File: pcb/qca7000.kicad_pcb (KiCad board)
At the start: 4 copper layers, 42.2 x 28.8 mm, 113 parts, among them J1 Conn_01x20, J2 JTAG, J3 FLASH, U1 AT25SF081-SSHD-X, Y1 25MHz

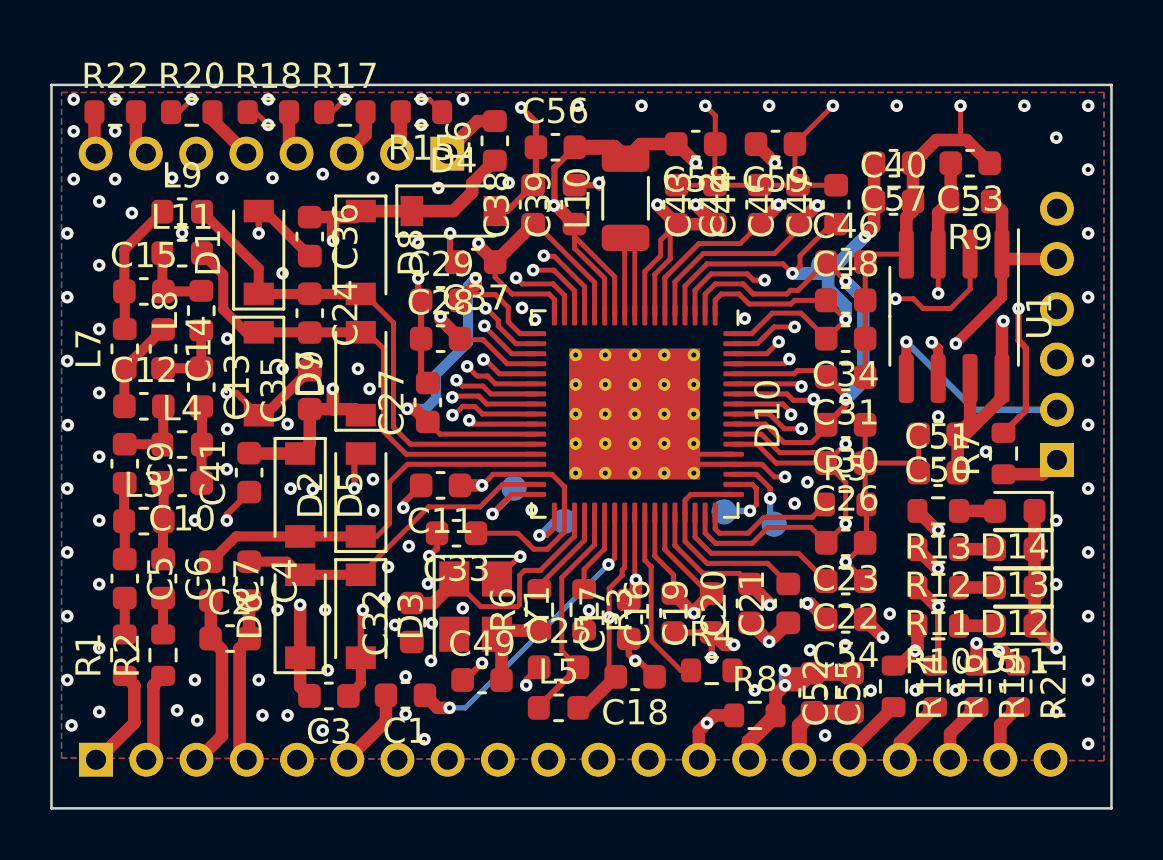
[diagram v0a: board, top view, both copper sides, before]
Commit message: v2, new filter, rbias
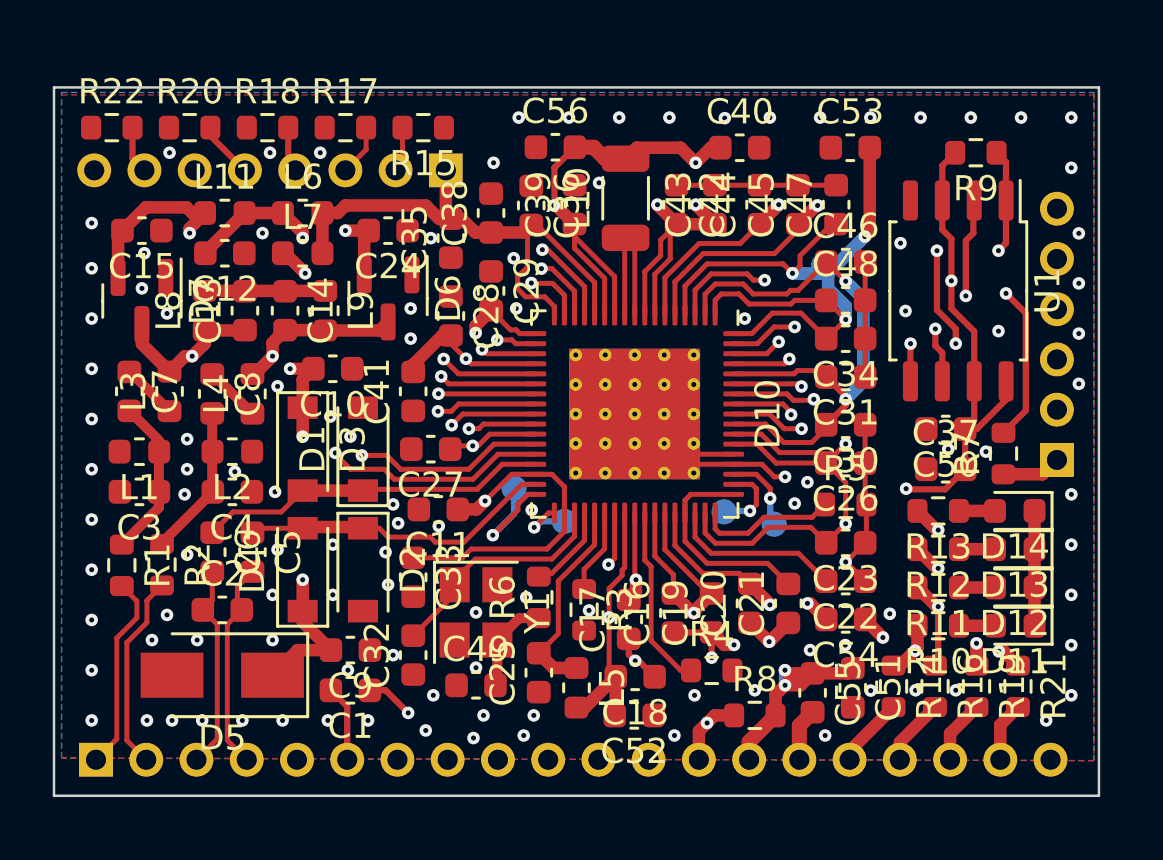
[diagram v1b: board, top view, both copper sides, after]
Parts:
- removed C57, C58, C59: 10uF 25V, Capacitor_SMD:C_0603_1608Metric
- removed D8, D9: 1N4148W, Diode_SMD:D_SOD-123
- added C8: 1.5nF, Capacitor_SMD:C_0603_1608Metric, F.Cu at (118.8, 61.0)
- added L1: 1.8uH, Inductor_SMD:L_0603_1608Metric, F.Cu at (115.9, 63.3)
- added L2: 1.8uH, Inductor_SMD:L_0603_1608Metric, F.Cu at (119.6, 63.3)
- C12, C35, C36, C37: value 100nF -> 10uF 25V
- C13, C14, C2, C3, C4: value 100nF -> 220pF
- C15, C24, C7: value 100nF -> 1.5nF
- C51: value 10uF 25V -> 100nF
- D1, D2, D3: value 1N4148W -> B5819W
- D4: value 4V7 -> B5819W
- D5: value 1N4148W -> 3V9; footprint Diode_SMD:D_SOD-123 -> Diode_SMD:D_SMA
- D6, D7: value 1N4148W -> BAV99; footprint Diode_SMD:D_SOD-123 -> Package_TO_SOT_SMD:SOT-23
- L11, L8, L9: value Bead 600 -> 1.8uH
- L3, L4: value Bead 600 -> 270nH
- R1, R2: value R_Small -> 22
- U1: value AT25SF081-SSHD-X -> 25Q16; footprint Package_SO:SOIC-8_3.9x4.9mm_P1.27mm -> Package_SO:SOP-8_5.28x5.23mm_P1.27mm
- moved C37 20.5 mm to (148.0, 64.0), turned to 0 degrees
- moved D4 15.5 mm to (122.4, 68.0), turned to 90 degrees
- moved D6 13.1 mm to (125.8, 57.2), turned to -90 degrees
- moved C9 11.7 mm to (124.3, 71.2), turned to 180 degrees
- moved C3 11.1 mm to (115.9, 64.9)
- moved C51 9.22 mm to (144.3, 72.7), turned to -90 degrees
- moved C36 8.90 mm to (131.5, 53.5)
- moved D1 8.86 mm to (124.8, 63.2)
- moved C52 8.72 mm to (135.6, 73.8), turned to 180 degrees
- moved C35 8.24 mm to (128.3, 54.8)
- moved C7 8.22 mm to (115.5, 60.9)
- moved L6 8.17 mm to (122.4, 53.8), turned to 0 degrees
- moved L7 8.04 mm to (122.4, 55.4), turned to 0 degrees
- moved D5 7.82 mm to (119.2, 72.2), turned to 180 degrees
- moved C10 7.52 mm to (123.6, 60.0)
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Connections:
- C10 pad 1: Net-(C10-Pad1) -> GND
- C11 pad 1: Net-(C11-Pad1) -> +3V3_A
- C12 pad 1: Net-(C12-Pad1) -> GND
- C12 pad 2: Net-(C12-Pad2) -> +3V3_A
- C13 pad 1: Net-(C13-Pad1) -> RXIN_N
- C13 pad 2: Net-(C10-Pad1) -> Net-(C13-Pad2)
- C14 pad 1: Net-(C12-Pad1) -> Net-(C13-Pad2)
- C14 pad 2: Net-(C13-Pad1) -> RXIN_P
- C15 pad 1: Net-(C15-Pad1) -> GND
- C24 pad 1: RXIN_N -> GND
- C24 pad 2: RXIN_P -> Net-(C15-Pad2)
- C3 pad 1: GND -> Net-(C3-Pad1)
- C3 pad 2: Net-(C11-Pad1) -> GND
- C33 pad 1: Net-(C11-Pad1) -> +3V3_A
- C35 pad 1: Net-(C11-Pad1) -> GND
- C35 pad 2: GND -> +3V3_D
- C36 pad 1: Net-(C11-Pad1) -> GND
- C36 pad 2: GND -> +3V3_D
- C37 pad 1: +3V3_D -> GND
- C37 pad 2: GND -> +3V3_D
- C4 pad 1: TXOUT_P -> GND
- C4 pad 2: TX_P -> Net-(C4-Pad2)
- C41 pad 2: Net-(C11-Pad1) -> +3V3_D
- C5 pad 1: Net-(C5-Pad1) -> TXOUT_P
- C5 pad 2: Net-(C5-Pad2) -> TX_P
- C51 pad 1: GND -> +3V3_D
- C51 pad 2: +3V3_D -> GND
- C52 pad 2: +3V3_D -> +1V2_C
- C53 pad 2: +3V3_D -> +1V2_C
- C6 pad 1: Net-(C10-Pad2) -> TXOUT_N
- C6 pad 2: Net-(C6-Pad2) -> TX_N
- C7 pad 1: TXOUT_N -> Net-(C7-Pad1)
- C7 pad 2: TX_N -> Net-(C3-Pad1)
- C9 pad 1: Net-(C12-Pad2) -> GND
- C9 pad 2: Net-(C5-Pad1) -> Net-(C10-Pad2)
- D1 pad 1: RXIN_N -> TXOUT_N
- D10 pad 32: Net-(C11-Pad1) -> +3V3_A
- D10 pad 36: Net-(C11-Pad1) -> +3V3_A
- D2 pad 1: TXOUT_N -> TXOUT_P
- D3 pad 1: TXOUT_P -> Net-(C10-Pad2)
- D3 pad 2: GND -> TXOUT_N
- D4 pad 1: Net-(C11-Pad1) -> Net-(C10-Pad2)
- D4 pad 2: GND -> TXOUT_P
- D5 pad 1: Net-(C11-Pad1) -> Net-(C10-Pad2)
- D5 pad 2: TXOUT_N -> GND
- D6 pad 1: Net-(C11-Pad1) -> GND
- D6 pad 2: TXOUT_P -> Net-(C15-Pad2)
- D7 pad 1: RXIN_P -> GND
- D7 pad 2: GND -> Net-(C15-Pad2)
- L11 pad 2: RXIN_P -> +3V3_A
- L3 pad 1: Net-(C5-Pad1) -> Net-(C7-Pad1)
- L3 pad 2: Net-(C10-Pad2) -> RXIN_N
- L4 pad 1: Net-(C12-Pad2) -> Net-(C8-Pad1)
- L4 pad 2: Net-(C10-Pad1) -> RXIN_P
- L6 pad 1: Net-(C11-Pad1) -> +3V3_A
- L7 pad 1: Net-(C12-Pad1) -> Net-(C10-Pad2)
- L7 pad 2: Net-(C15-Pad1) -> +3V3_D
- L8 pad 1: Net-(C13-Pad1) -> RXIN_N
- L8 pad 2: Net-(C15-Pad2) -> Net-(C13-Pad2)
- L9 pad 1: Net-(C15-Pad1) -> Net-(C13-Pad2)
- L9 pad 2: RXIN_N -> RXIN_P
- R1 pad 1: RX_N -> Net-(C3-Pad1)
- R1 pad 2: Net-(C5-Pad2) -> RX_N
- R2 pad 1: RX_P -> Net-(C4-Pad2)
- R2 pad 2: Net-(C6-Pad2) -> RX_P
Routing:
- net GND: track 117.3 -> 45.2 mm, vias 137 -> 115
- net Net-(C11-Pad1): track 53.1 -> 0.00 mm, vias 4 -> 0
- net +3V3_A: track 0.00 -> 32.5 mm, vias 0 -> 2
- net Net-(C10-Pad2): track 3.06 -> 20.9 mm, vias 0 -> 4
- net Net-(C15-Pad2): track 3.06 -> 16.3 mm, vias 0 -> 2
- net +3V3_D: track 157.2 -> 168.5 mm, vias 13 -> 12
- net Net-(C3-Pad1): track 0.00 -> 6.43 mm
- net Net-(C4-Pad2): track 0.00 -> 6.05 mm
- net Net-(C15-Pad1): track 5.30 -> 0.00 mm
- net Net-(C13-Pad2): track 0.00 -> 4.80 mm
- net RX_P: track 3.62 -> 7.84 mm
- net SPI_CS_L: track 18.1 -> 22.3 mm, vias 2 -> 4
- net RXIN_P: track 19.4 -> 23.4 mm, vias 0 -> 2
- net Net-(C12-Pad1): track 3.70 -> 0.00 mm
- net RX_N: track 4.17 -> 7.84 mm
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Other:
- board size 42.2 x 28.8 mm -> 41.6 x 28.2 mm
